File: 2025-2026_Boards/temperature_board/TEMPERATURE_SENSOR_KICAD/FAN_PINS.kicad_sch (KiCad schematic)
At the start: 27 parts, among them J10 Conn_01x02_Pin, J11 Conn_01x02_Pin, J12 Conn_01x02_Pin, J13 Conn_01x02_Pin, J14 Conn_01x02_Pin, J15 Conn_01x02_Pin, J16 Conn_01x02_Pin, J17 Conn_01x02_Pin, J18 Conn_01x02_Pin, J19 Conn_01x02_Pin, J2 Conn_01x02_Pin, J20 Conn_01x02_Pin, J21 Conn_01x02_Pin, J22 Conn_01x02_Pin, J23 Conn_01x02_Pin, J24 Conn_01x03_Socket, J25 Conn_01x03_Socket, J3 Conn_01x02_Pin, J4 Conn_01x02_Pin, J5 Conn_01x02_Pin, J6 Conn_01x02_Pin, J7 Conn_01x02_Pin, J8 Conn_01x02_Pin, J9 Conn_01x02_Pin, U4 TCAN1057AEV-Q1

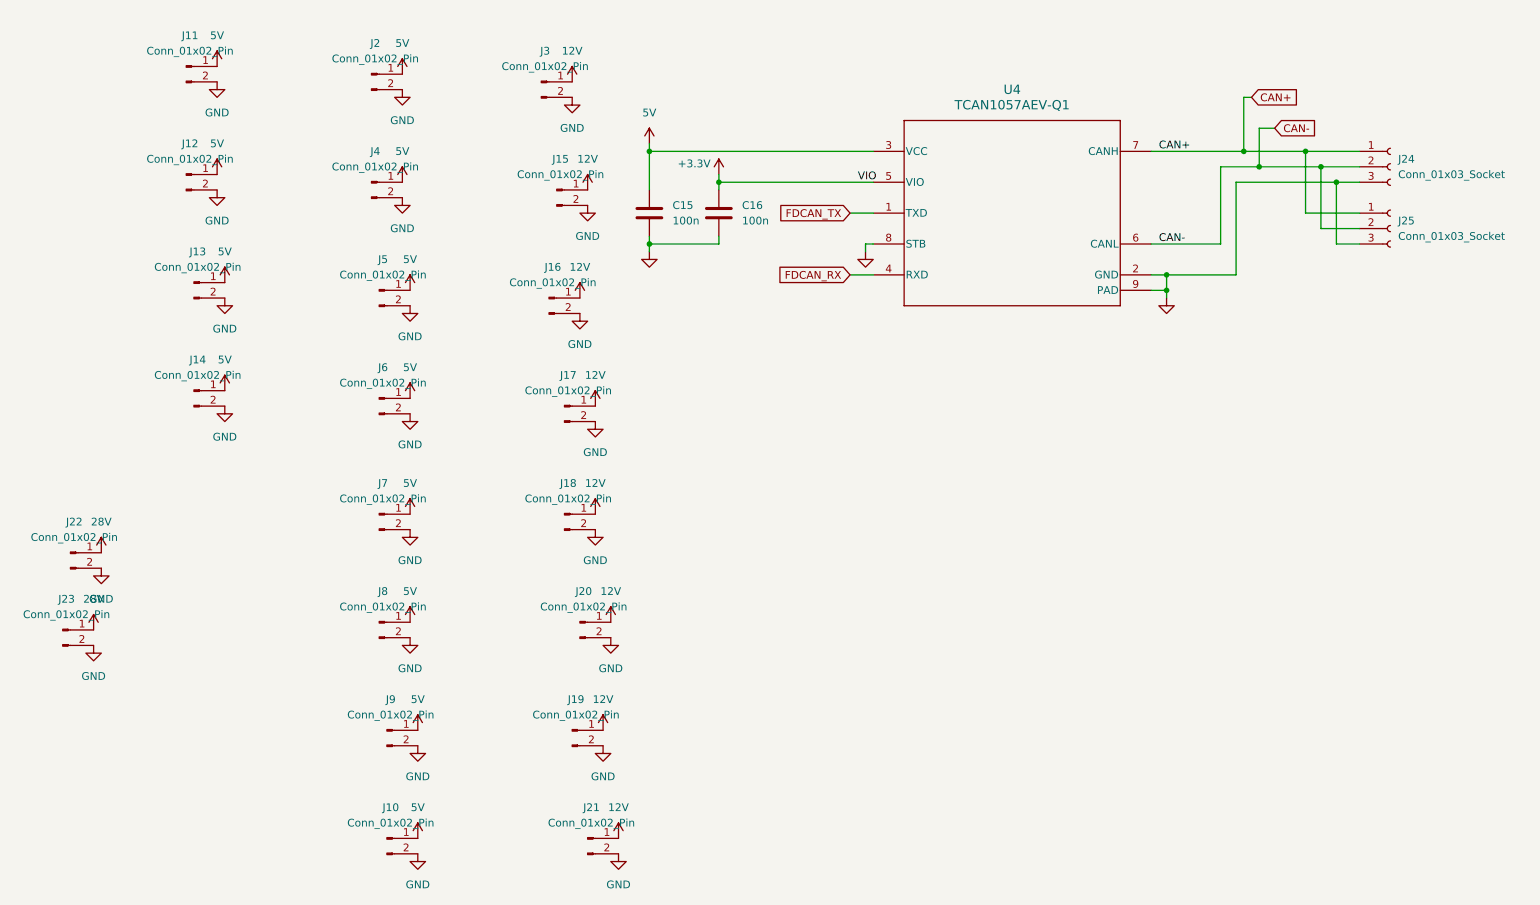
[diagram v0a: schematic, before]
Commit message: finalizing board
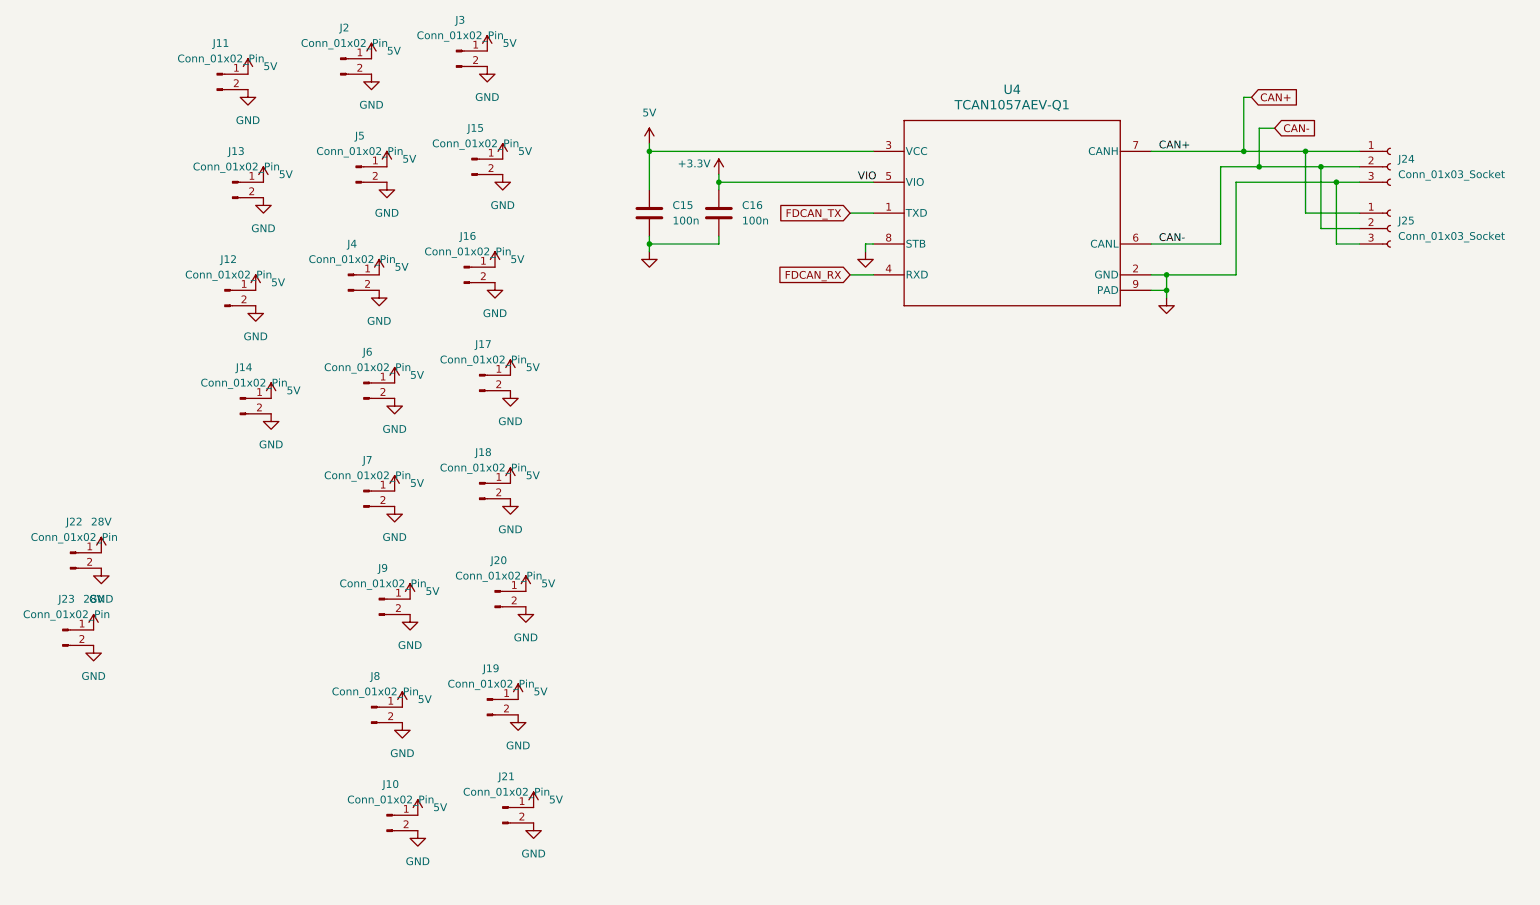
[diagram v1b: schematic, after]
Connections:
- net 12V is gone; now on net 5V: J15.1 (Pin_1), J16.1 (Pin_1), J17.1 (Pin_1), J18.1 (Pin_1), J19.1 (Pin_1), J20.1 (Pin_1), J21.1 (Pin_1), J3.1 (Pin_1)
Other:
- moved on the sheet: J15, J16, J17, J18, J19, J20, J21, J3
